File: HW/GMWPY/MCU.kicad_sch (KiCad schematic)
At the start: 27 parts, among them J2 Micro_SD_Card_Det, SW1 MCU_RESET, SW2 MCU_RESET, U11 ESP32-S3-WROOM-1

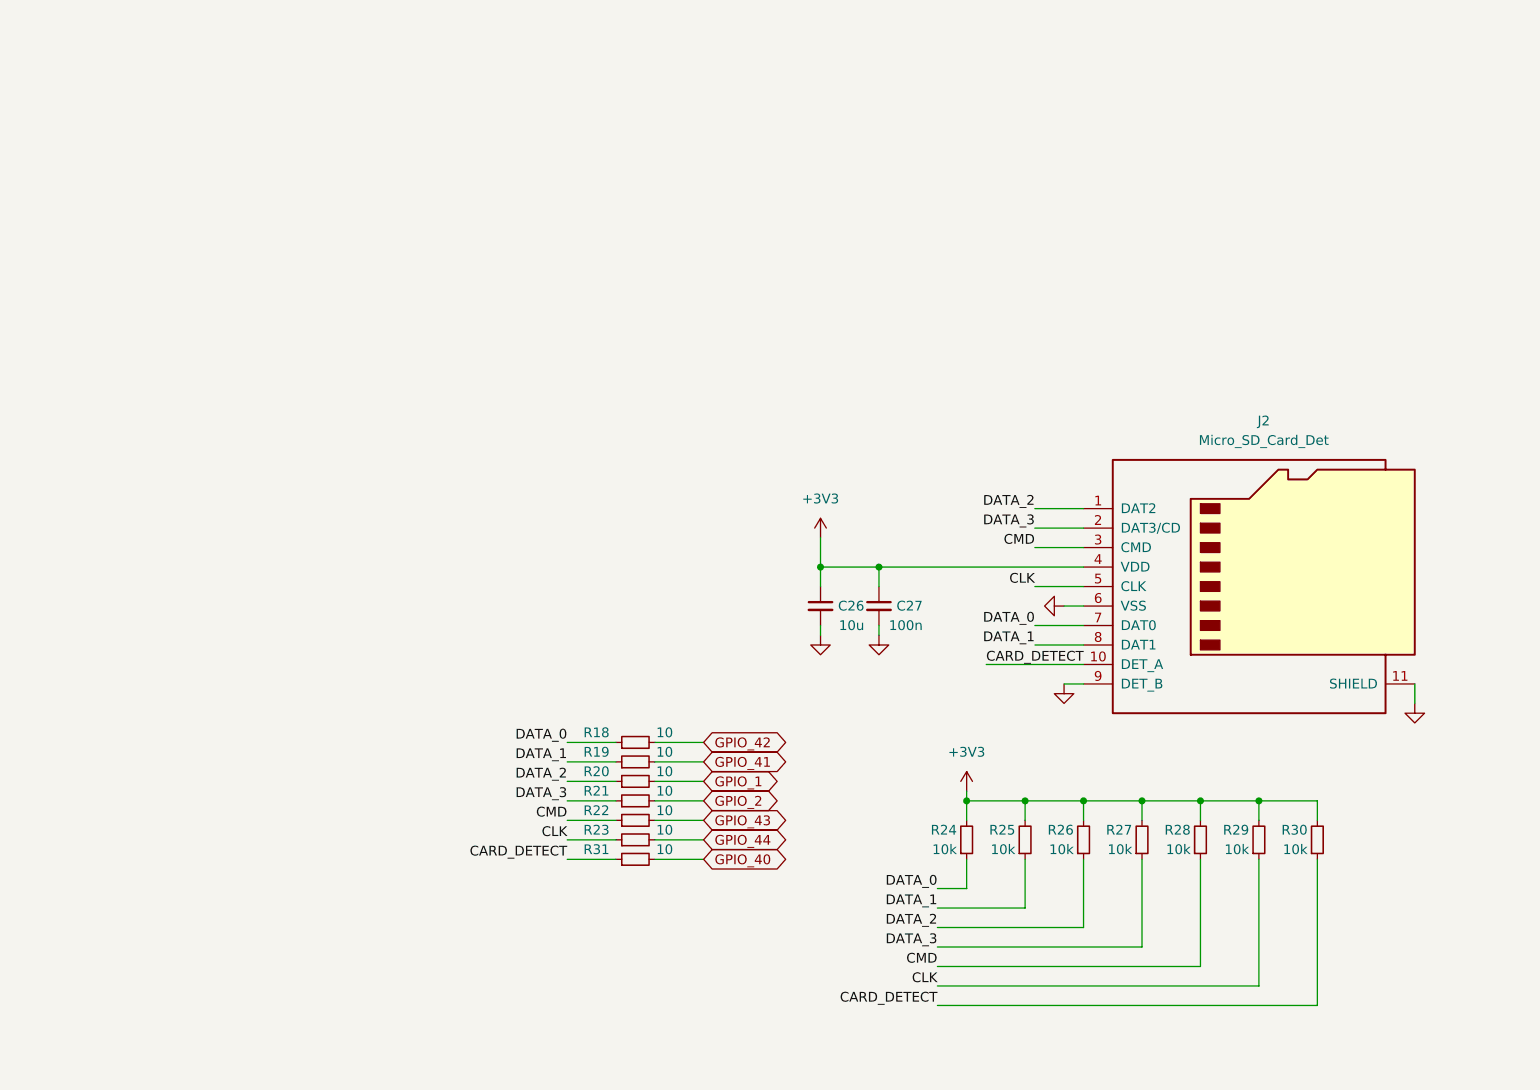
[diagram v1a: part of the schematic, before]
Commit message: G
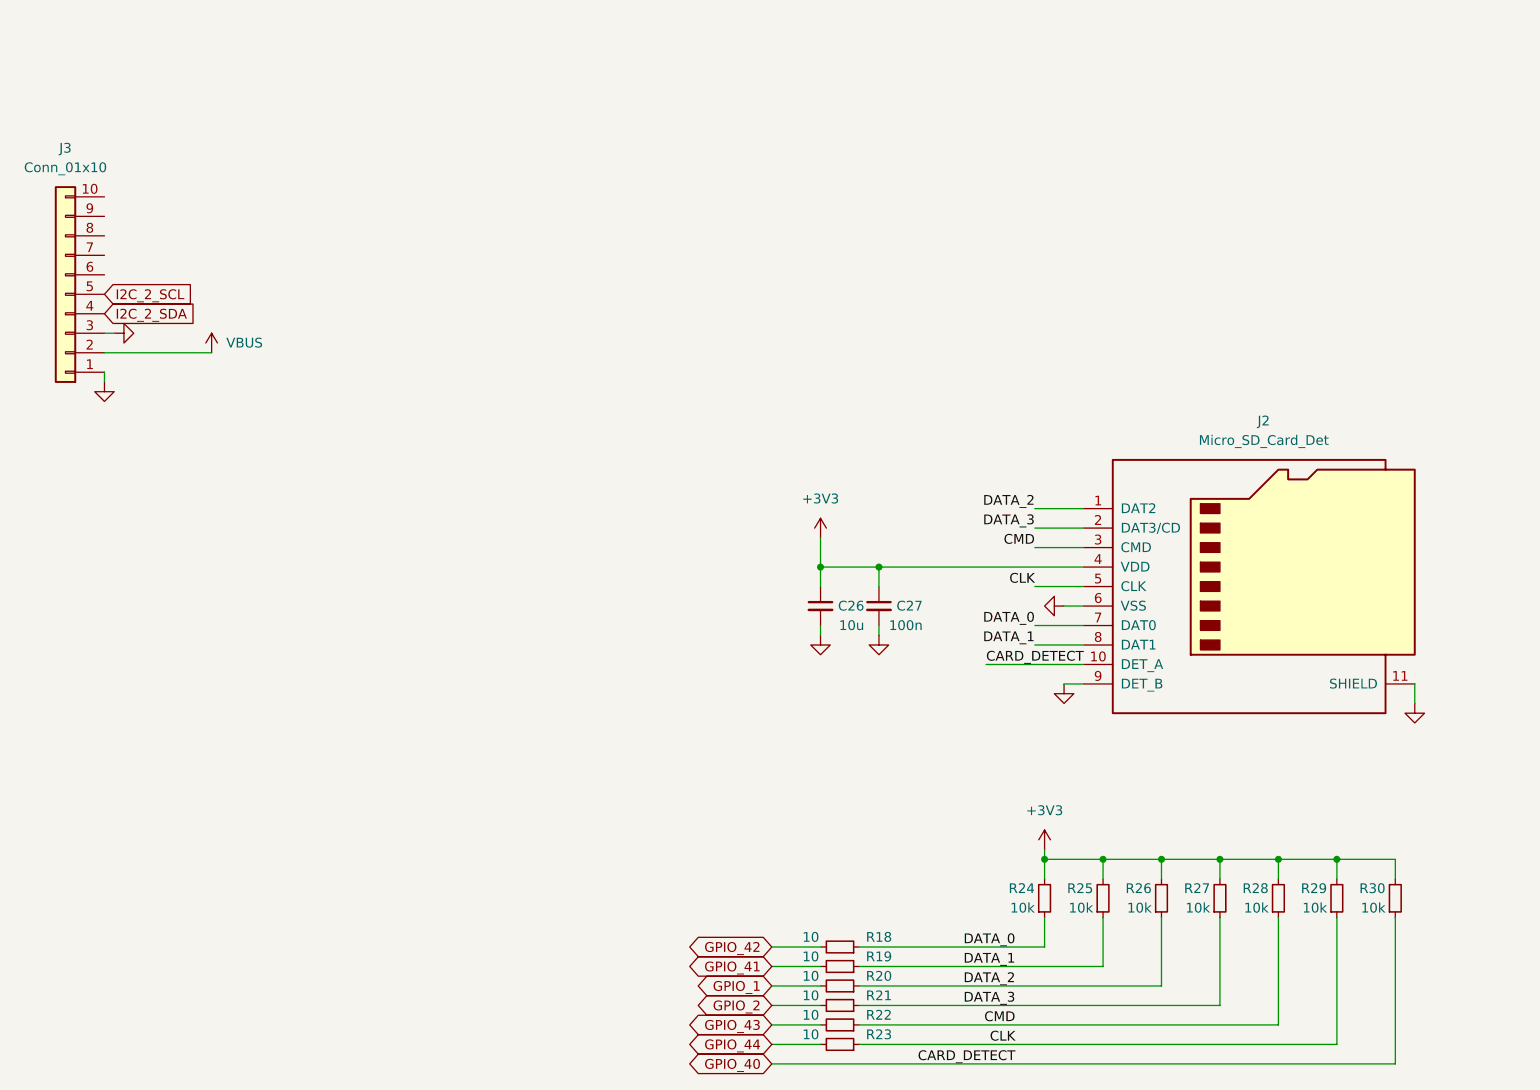
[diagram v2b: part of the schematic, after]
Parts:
- removed R31: 10, Resistor_SMD:R_0402_1005Metric, symbol Device:R_Small
- added J3: Conn_01x10, symbol Connector_Generic:Conn_01x10
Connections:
- net CARD_DETECT is gone; now on net GPIO_40: J2.10 (DET_A), R30.1
- net GND: now also J3.1 (Pin_1), J3.3 (Pin_3)
- new net I2C_2_SCL: J3.5 (Pin_5)
- new net I2C_2_SDA: J3.4 (Pin_4)
- new net VBUS: J3.2 (Pin_2)
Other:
- moved on the sheet: R18, R19, R20, R21, R22, R23, R24, R25, R26, R27, R28, R29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

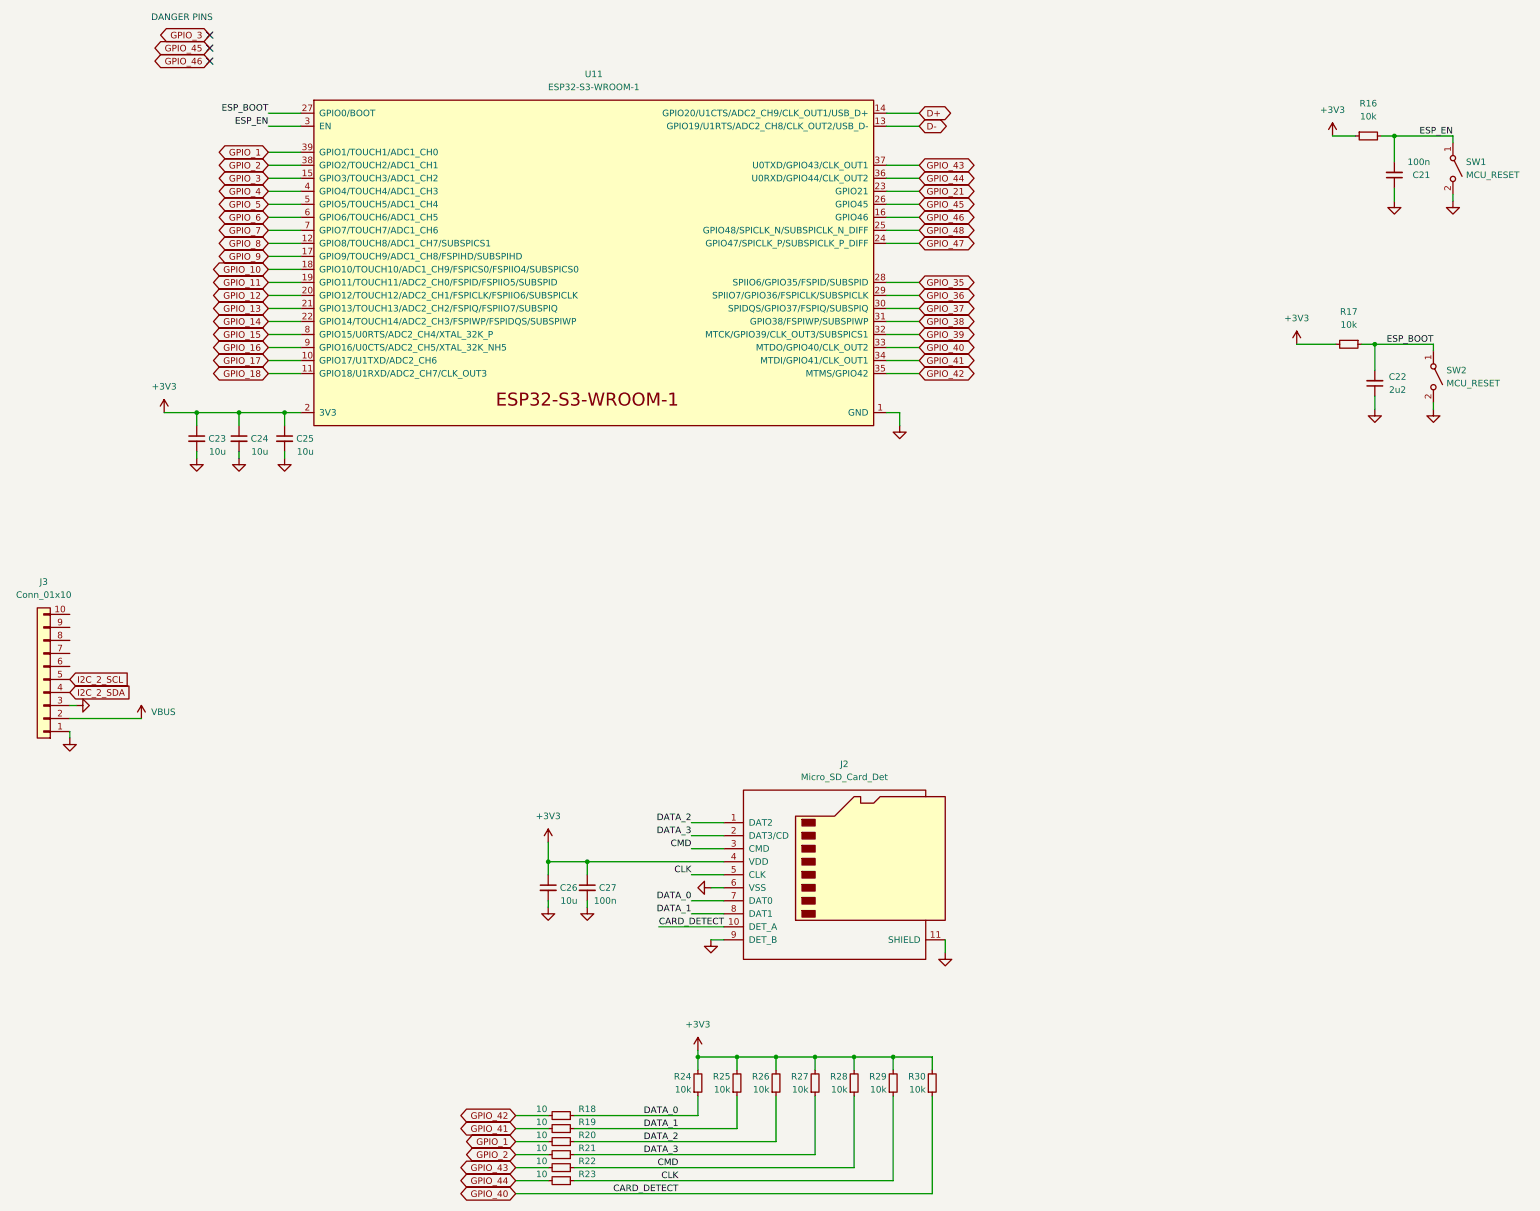
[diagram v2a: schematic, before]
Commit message: n
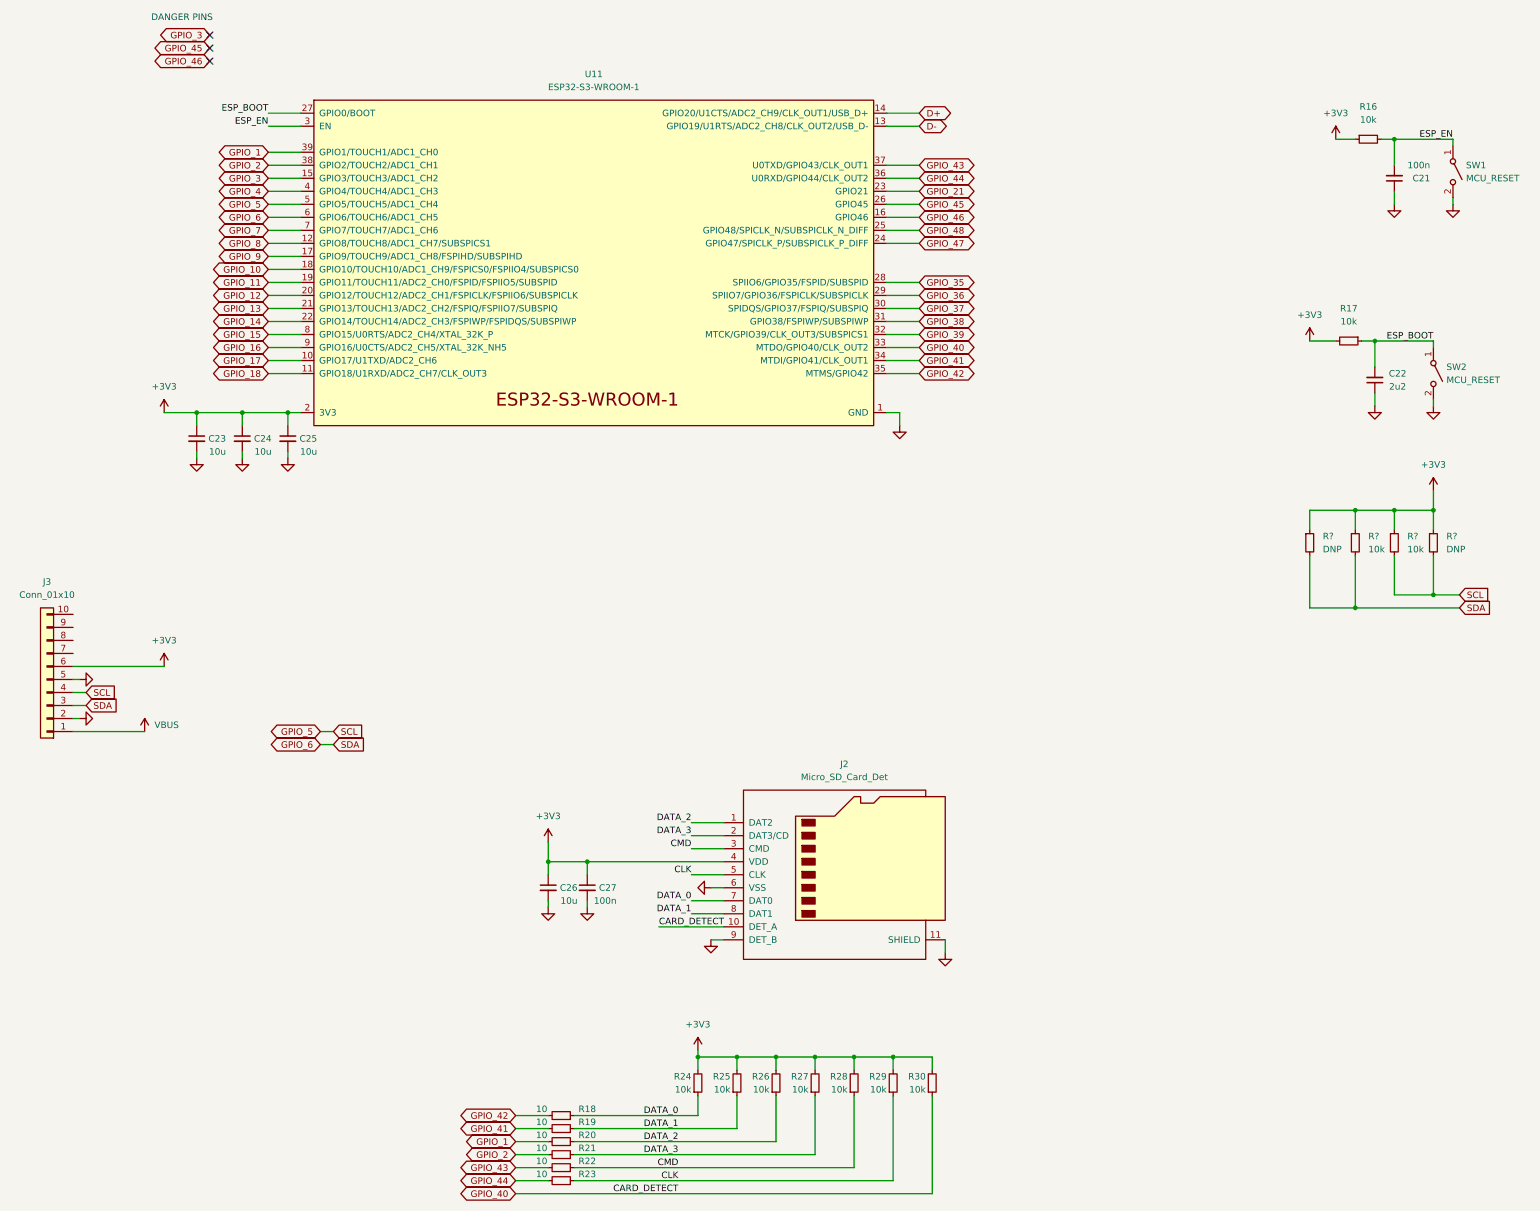
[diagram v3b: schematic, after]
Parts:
- added R? (x2): DNP, Resistor_SMD:R_0603_1608Metric_Pad0.98x0.95mm_HandSolder, symbol Device:R_Small
- added R? (x2): 10k, Resistor_SMD:R_0603_1608Metric_Pad0.98x0.95mm_HandSolder, symbol Device:R_Small
- J3: footprint (none) -> Connector_PinHeader_2.54mm:PinHeader_1x06_P2.54mm_Vertical; now left out of the parts list
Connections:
- net I2C_2_SCL is gone; now on net GND: J3.5 (Pin_5)
- net I2C_2_SDA is gone; now on net GPIO_5: J3.4 (Pin_4)
- net +3V3: now also J3.6 (Pin_6), R?.1, R?.1, R?.1, R?.1
- net GND: now also J3.2 (Pin_2); no longer J3.1 (Pin_1), J3.3 (Pin_3)
- net GPIO_5: now also R?.2, R?.2
- net GPIO_6: now also J3.3 (Pin_3), R?.2, R?.2
- net VBUS: now also J3.1 (Pin_1); no longer J3.2 (Pin_2)
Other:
- moved on the sheet: C21, C22, C24, C25, J3, R16, R17, SW1, SW2
